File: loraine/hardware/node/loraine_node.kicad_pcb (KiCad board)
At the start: 2 copper layers, 50 x 50 mm, 46 parts, among them CON1 BARREL_JACK, IC1 ATTINY2313A-S, K1 LED1, K2 LED2, K3 LED3, P1 POWER_THRU, P2 POWER, P3 SOLDER_PAD, P4 BUS, P5 BUS_THRU, P6 ICSP, P7 OUTPUTS, Q1 TSM3460CX6, Q2 TSM3460CX6, Q3 TSM3460CX6, Q4 TSM3460CX6, Q5 TSM3460CX6, Q6 TSM3460CX6, Q7 TSM3460CX6, Q8 TSM3460CX6, U1 UA7805CKCT, U2 SN65176BD, X1 16MHz

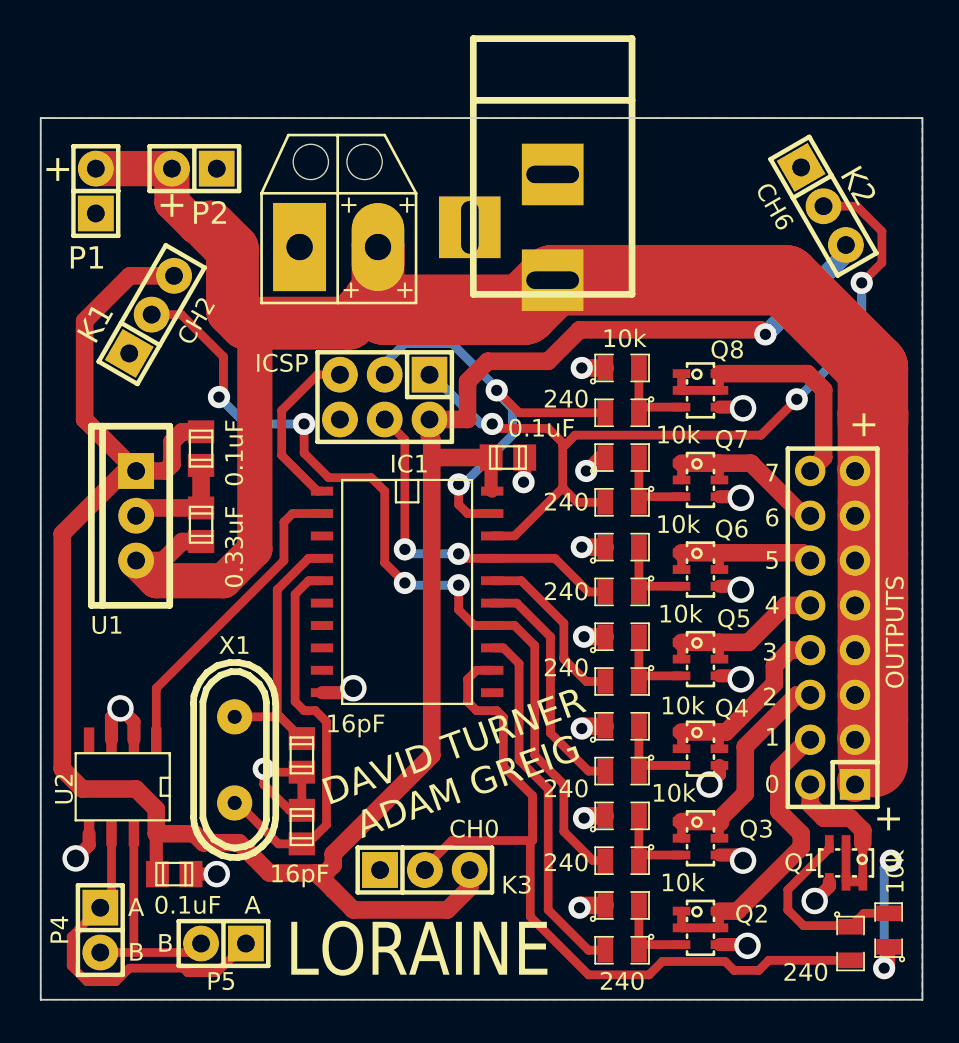
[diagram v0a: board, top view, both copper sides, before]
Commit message: Adam's changes and gerbils
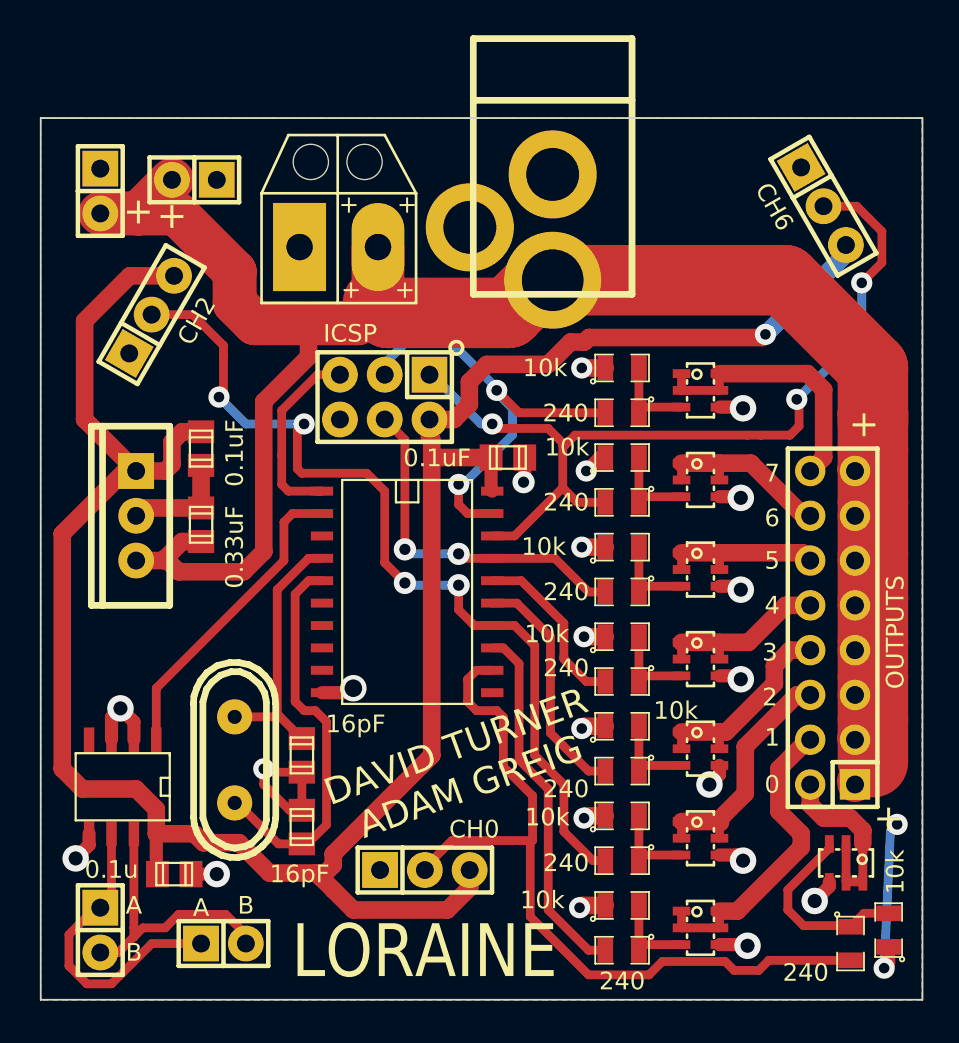
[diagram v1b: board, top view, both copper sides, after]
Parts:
- C4: value 0.1uF -> 0.1u
- moved P2 0.63 mm to (108.7, 103.5)
- moved P1 0.25 mm to (103.4, 104.1), turned to 270 degrees
- turned P5 to 0 degrees
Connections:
- CON1 pad 3: (no net) -> GND
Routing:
- net /B: track 12.7 -> 16.6 mm
- net GND: track 52.9 -> 55.0 mm
- net /A: track 19.8 -> 18.2 mm
- net /LED2: track 49.7 -> 51.2 mm
- net /RESET: track 9.81 -> 11.0 mm
- net /LED6: track 49.6 -> 50.7 mm
- net +5V: track 136.7 -> 136.0 mm
- net VIN: track 117.9 -> 117.3 mm
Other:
- rule via_min_drill: 0.508 -> 0.6
- rule via_min_size: 1.26 -> 1.2
